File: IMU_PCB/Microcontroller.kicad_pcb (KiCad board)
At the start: 2 copper layers, 100 x 64.2 mm, 28 parts, among them J1 Conn_01x02, J4 Conn_01x02_Pin, U1 TPS54560BQDDARQ1, U10 Thermal Resistor, U2 ESP32-DEVKIT-C, U6 TJA1050T/CM,118, U7 Adafruit ICM-20948, U8 SDIO Card Breakout Board, U9 AM2302

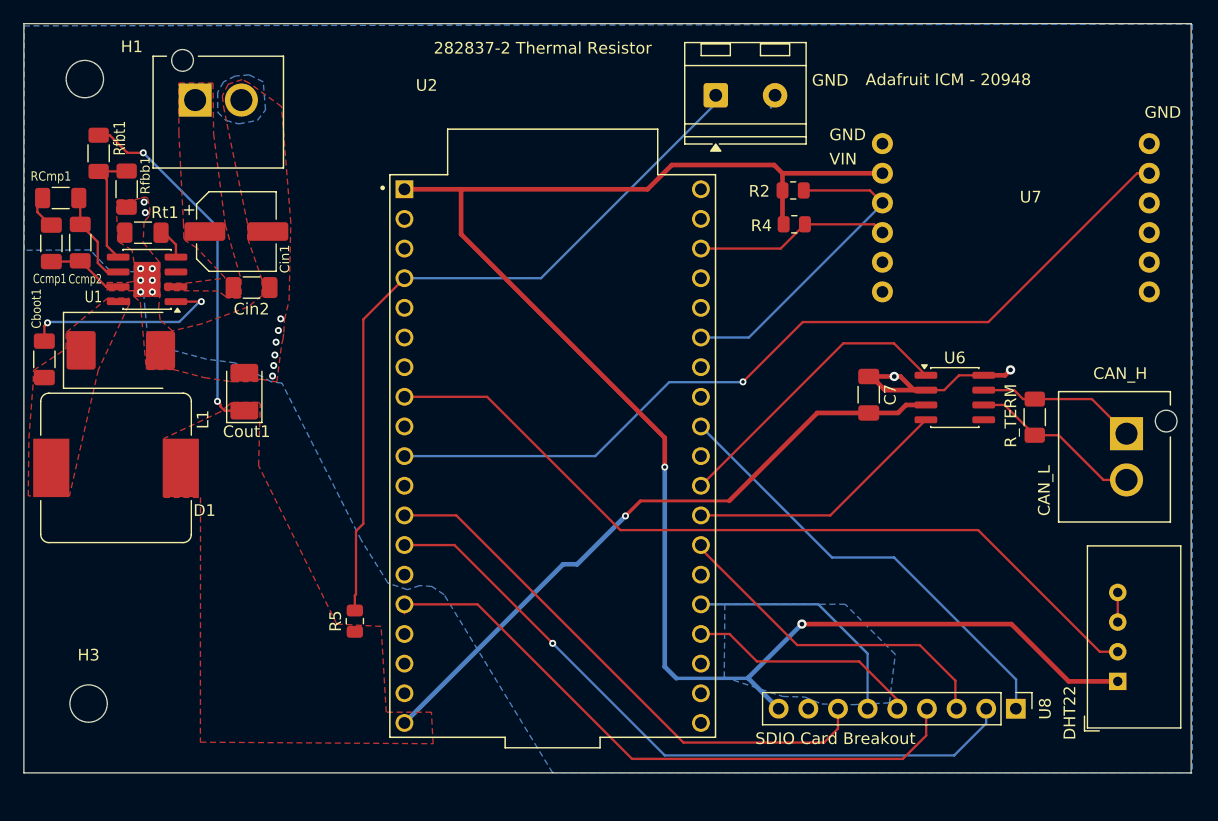
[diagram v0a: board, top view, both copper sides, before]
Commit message: PDB_Schematic mostly updated
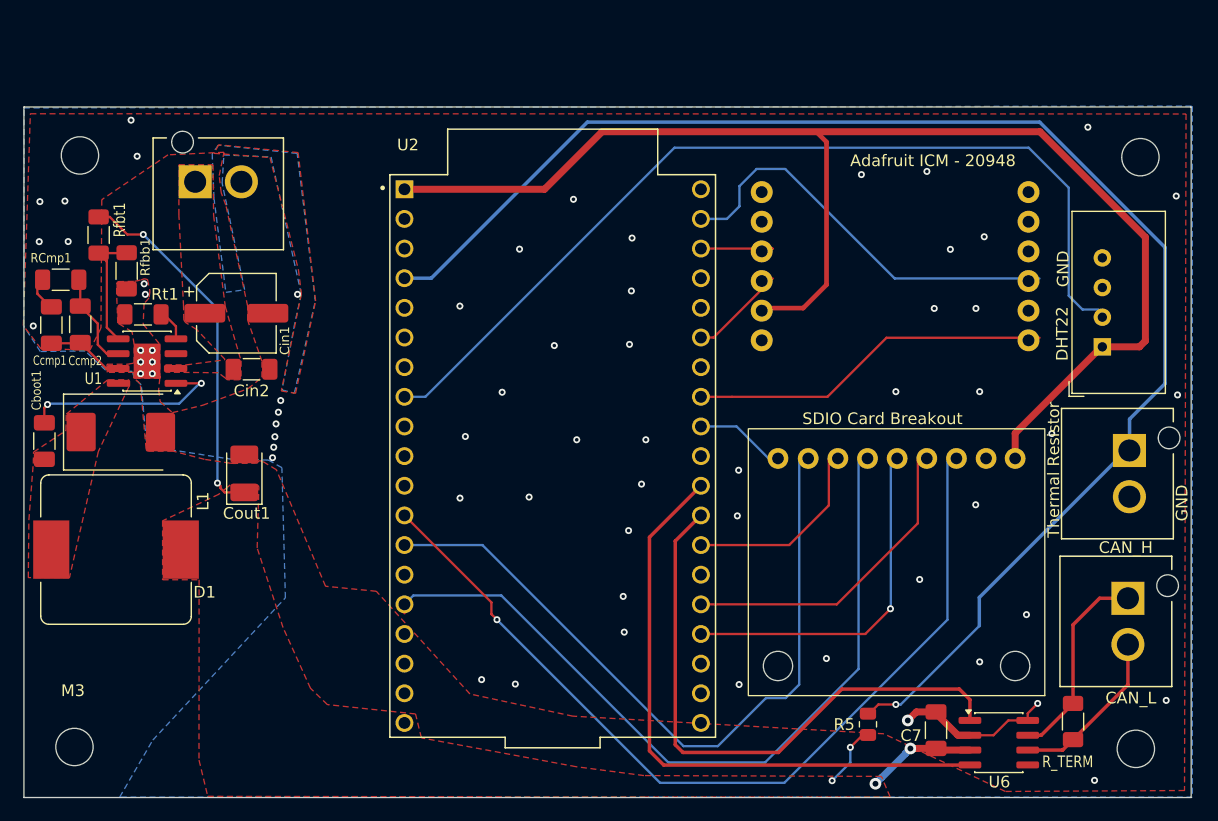
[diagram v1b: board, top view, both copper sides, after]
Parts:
- removed R2, R4: 10k, Resistor_SMD:R_0805_2012Metric
- added H2: MountingHole, MountingHole:MountingHole_3.2mm_M3, F.Cu at (196.2, 56.2)
- added H4: MountingHole, MountingHole:MountingHole_3.2mm_M3, F.Cu at (195.8, 106.9)
- U10: footprint TerminalBlock_RND:TerminalBlock_RND_205-00232_1x02_P5.08mm_Horizontal -> PROVE-footprints:TE_1877285-2
- U7: value Adafruit ICM-20948 -> SparkFun: ISM330DHCX, MMC5983MA; footprint PROVE-footprints:Adafruit_ICM20948_2x6_Module -> PROVE-footprints:SparkFun 9DoF IMU Breakout - ISM330DHCX, MMC5983MA (Qwiic); moved to B.Cu
- U8: footprint Connector_PinHeader_2.54mm:PinHeader_1x09_P2.54mm_Vertical -> PROVE-footprints:Adafruit SDIO card breakout
- moved U10 47.3 mm to (194.2, 83.4), turned to -90 degrees
- moved R5 44.8 mm to (172.8, 104.8)
- moved U6 29.8 mm to (184.0, 106.4)
- moved C7 29.3 mm to (178.6, 105.3)
- moved U9 28.7 mm to (192.9, 72.5)
- moved R8 26.3 mm to (190.4, 104.6)
- moved U7 15.8 mm to (188.0, 78.4), turned to 90 degrees
- moved J4 14.1 mm to (194.1, 96.0)
- moved Cin1 7.00 mm to (118.7, 69.6)
- moved Cboot1 7.00 mm to (102.2, 80.6)
- moved Cin2 7.00 mm to (120.0, 74.4)
- moved Cout1 7.00 mm to (119.4, 83.3)
- moved D1 7.00 mm to (108.8, 79.8)
- moved J1 7.00 mm to (117.2, 59.4)
- moved L1 7.00 mm to (108.4, 89.9)
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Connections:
- U2 pad 10: Net-(U2-IO26) -> unconnected-(U2-IO26-Pad10)
- U2 pad 31: unconnected-(U2-IO19-Pad31) -> Net-(U2-IO19)
- U2 pad 37: unconnected-(U2-IO23-Pad37) -> Net-(U2-IO23)
- U6 pad 1: Net-(U2-IO17) -> Net-(U2-IO16)
- U6 pad 4: Net-(U2-IO16) -> Net-(U2-IO17)
- U7 pad 1: GND -> Net-(U2-IO19)
- U7 pad 10: unconnected-(U7-Pin_10-Pad10) -> Net-(U2-IO21)
- U7 pad 11: Net-(U2-IO26) -> Net-(U2-3V3)
- U7 pad 2: Net-(U2-3V3) -> unconnected-(U7-Pin_2-Pad2)
- U7 pad 3: Net-(U2-IO21) -> Net-(U2-IO23)
- U7 pad 4: Net-(U2-IO22) -> unconnected-(U7-Pin_4-Pad4)
- U7 pad 9: unconnected-(U7-Pin_9-Pad9) -> Net-(U2-IO22)
- U8 pad 1: Net-(U2-IO18) -> Net-(U2-3V3)
- U8 pad 2: Net-(U2-IO12) -> GND
- U8 pad 3: Net-(U2-IO4) -> Net-(U2-IO14)
- U8 pad 4: Net-(U2-IO13) -> Net-(U2-IO2)
- U8 pad 6: Net-(U2-IO2) -> Net-(U2-IO13)
- U8 pad 7: Net-(U2-IO14) -> Net-(U2-IO4)
- U8 pad 8: GND -> Net-(U2-IO12)
- U8 pad 9: Net-(U2-3V3) -> Net-(U2-IO18)
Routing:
- net Net-(U2-IO26): track 73.9 -> 0.00 mm, vias 1 -> 0
- net Net-(U10-Pin_1): track 64.0 -> 126.8 mm, vias 0 -> 1
- net /BUCK_5V: track 86.8 -> 46.0 mm, vias 3 -> 6
- net Net-(U2-IO23): track 0.00 -> 35.7 mm
- net Net-(U2-3V3): track 146.4 -> 113.7 mm, vias 2 -> 0
- net Net-(U2-IO19): track 0.00 -> 31.2 mm
- net Net-(U2-IO18): track 38.4 -> 7.73 mm
- net Net-(U2-IO14): track 47.7 -> 76.5 mm, vias 0 -> 1
- net Net-(U2-IO16): track 22.7 -> 50.5 mm
- net Net-(U2-IO17): track 25.5 -> 52.5 mm
- net Net-(U2-IO21): track 27.6 -> 8.24 mm
- net Net-(U2-IO13): track 54.1 -> 67.2 mm
- net Net-(U2-IO4): track 29.2 -> 16.6 mm
- net Net-(U2-IO22): track 16.7 -> 6.16 mm
- net Net-(U2-IO15): track 19.9 -> 29.8 mm, vias 0 -> 1
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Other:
- board size 100 x 64.2 mm -> 100 x 59.2 mm
- board text added: "M3"
- board text removed: "282837-2 Thermal Resistor"
